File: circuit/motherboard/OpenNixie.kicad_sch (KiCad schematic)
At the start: 29 parts, among them J1 Jack-DC, J2 Nixie_Conn_12P, J3 Nixie_Conn_12P, J4 Nixie_Conn_12P, J5 Nixie_Conn_12P, J6 Conn_01x05, Q1 MPSA42, Q2 TK8P65W, U1 AMS1117, U2 MAX1771CSA, U3 74HC595, U4 74HC595

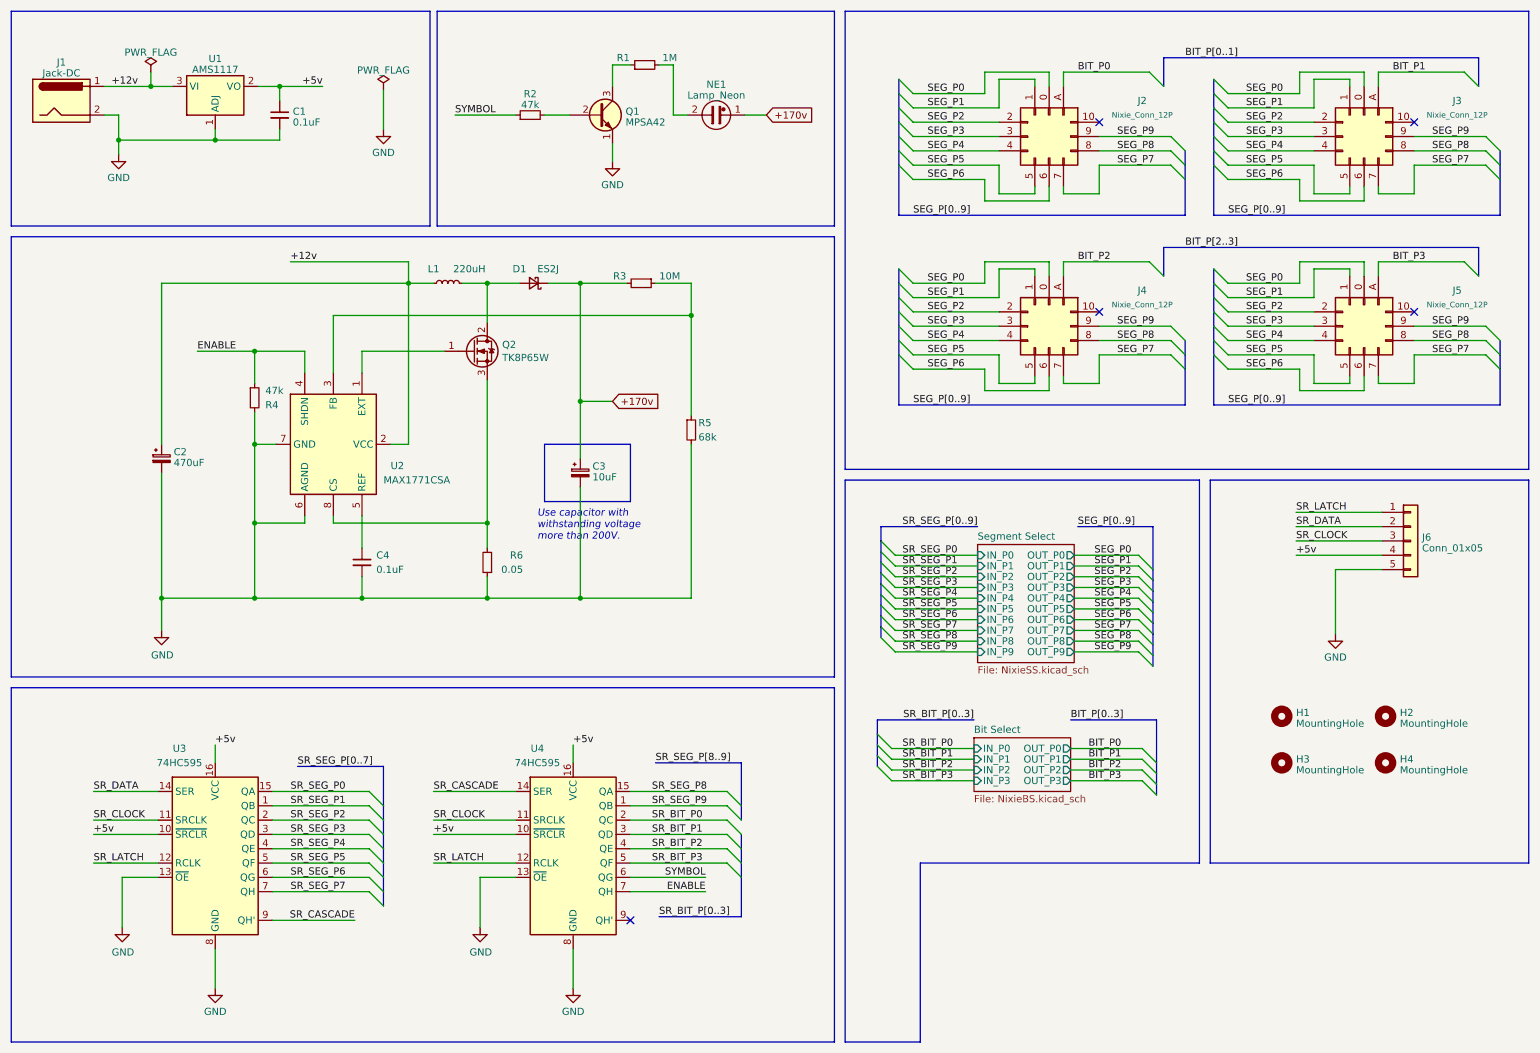
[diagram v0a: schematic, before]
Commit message: Some integration works
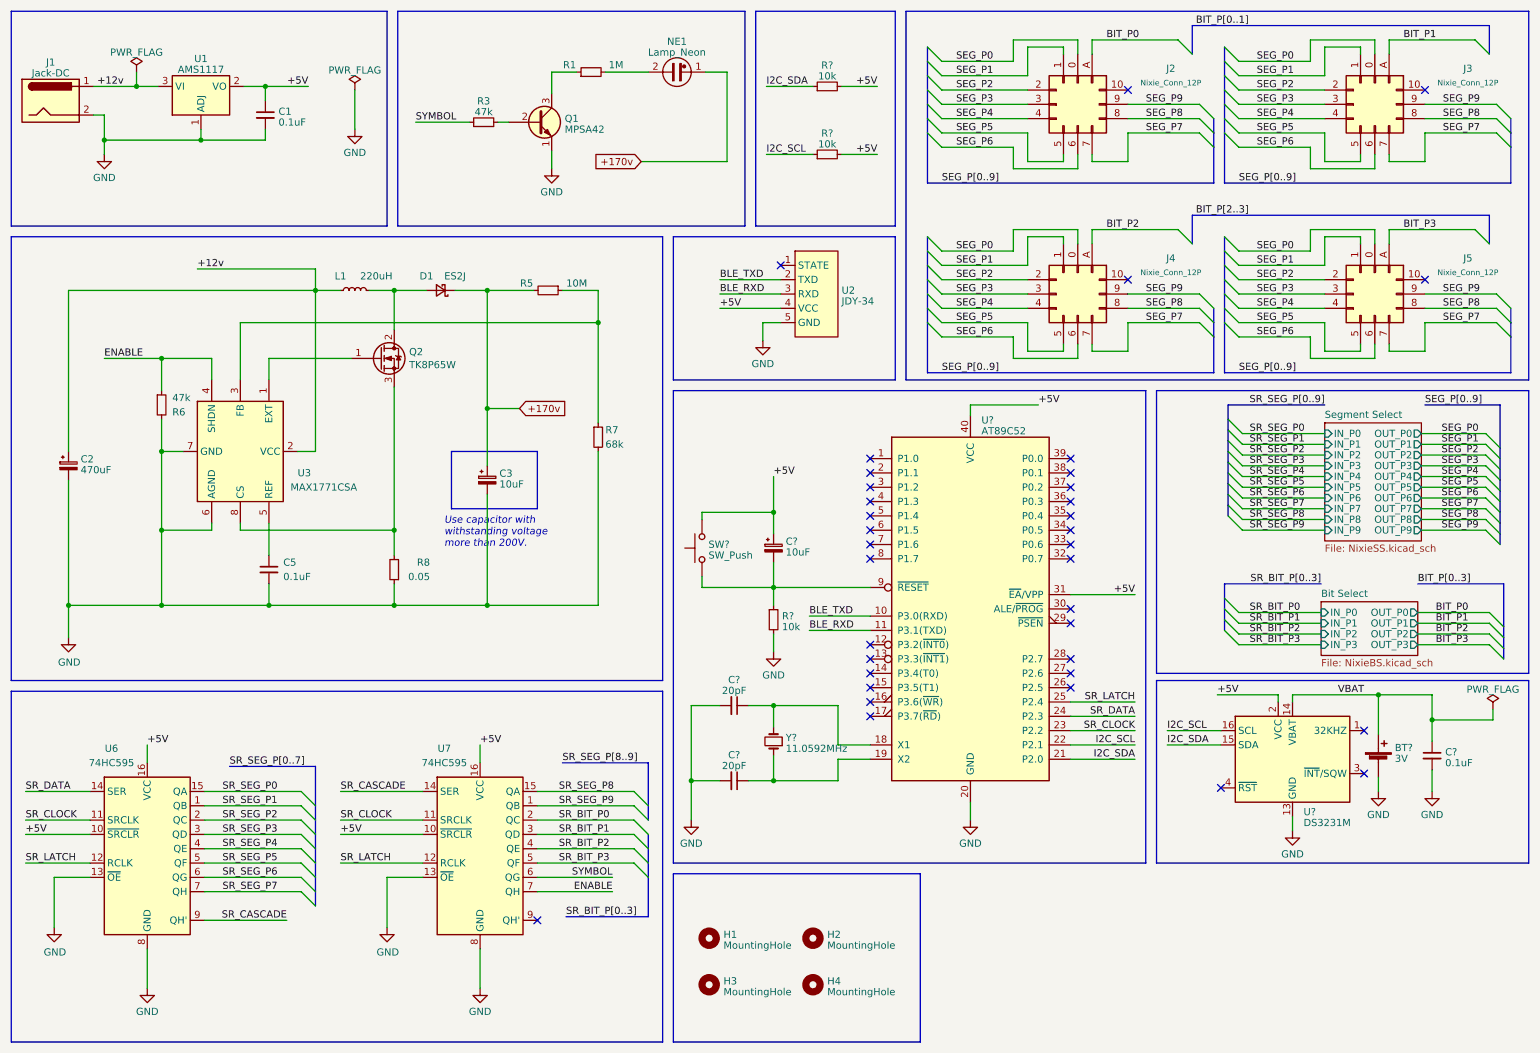
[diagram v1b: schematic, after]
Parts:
- removed J6: Conn_01x05, Connector_PinHeader_2.54mm:PinHeader_1x05_P2.54mm_Vertical, symbol Connector_Generic:Conn_01x05
- added BT?: 3V, Battery:BatteryHolder_LINX_BAT-HLD-012-SMT, symbol Device:Battery_Cell
- added C? (x2): 20pF, Capacitor_THT:C_Disc_D3.0mm_W2.0mm_P2.50mm, symbol Device:C_Small
- added C?: 10uF, Capacitor_THT:CP_Radial_D5.0mm_P2.50mm, symbol Device:C_Polarized_Small
- added C?: 0.1uF, Capacitor_THT:C_Disc_D3.0mm_W2.0mm_P2.50mm, symbol Device:C_Small
- added R? (x3): 10k, Resistor_THT:R_Axial_DIN0204_L3.6mm_D1.6mm_P7.62mm_Horizontal, symbol Device:R_Small
- added SW?: SW_Push, Button_Switch_SMD:SW_SPST_FSMSM, symbol Switch:SW_Push
- added U2: JDY-34, Connector_PinSocket_2.54mm:PinSocket_1x05_P2.54mm_Vertical, symbol Nixie_Clock:JDY-34
- added U?: AT89C52, Package_DIP:DIP-40_W15.24mm, symbol Nixie_Clock:AT89C52
- added U?: DS3231M, Package_SO:SOIC-16W_7.5x10.3mm_P1.27mm, symbol Timer_RTC:DS3231M
- added Y?: 11.0592MHz, Crystal:Crystal_HC18-U_Vertical, symbol Device:Crystal_Small
- R1: footprint Resistor_THT:R_Axial_DIN0204_L3.6mm_D1.6mm_P5.08mm_Horizontal -> Resistor_THT:R_Axial_DIN0204_L3.6mm_D1.6mm_P7.62mm_Horizontal
- R3: renamed from R2; footprint Resistor_THT:R_Axial_DIN0204_L3.6mm_D1.6mm_P5.08mm_Horizontal -> Resistor_THT:R_Axial_DIN0204_L3.6mm_D1.6mm_P7.62mm_Horizontal
- R5: renamed from R3; footprint Resistor_THT:R_Axial_DIN0204_L3.6mm_D1.6mm_P5.08mm_Horizontal -> Resistor_THT:R_Axial_DIN0204_L3.6mm_D1.6mm_P7.62mm_Horizontal
- R6: renamed from R4; footprint Resistor_THT:R_Axial_DIN0204_L3.6mm_D1.6mm_P5.08mm_Horizontal -> Resistor_THT:R_Axial_DIN0204_L3.6mm_D1.6mm_P7.62mm_Horizontal
- R7: renamed from R5; footprint Resistor_THT:R_Axial_DIN0204_L3.6mm_D1.6mm_P5.08mm_Horizontal -> Resistor_THT:R_Axial_DIN0204_L3.6mm_D1.6mm_P7.62mm_Horizontal
- renumbered C4 to C5, R6 to R8, U2 to U3, U3 to U6, U4 to U7
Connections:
- net GND: now also BT?.2 (-), C?.2, C?.2, C?.2, R?.2, U2.5 (GND), U?.10 (GND), U?.11 (GND), U?.12 (GND), U?.13 (GND), U?.20 (GND), U?.5 (GND), U?.6 (GND), U?.7 (GND), U?.8 (GND), U?.9 (GND)
- net SR_CLOCK: now also U?.23 (P2.2)
- net SR_DATA: now also U?.24 (P2.3)
- net SR_LATCH: now also U?.25 (P2.4)
- net +5v renamed +5V
- net +5V: now also C?.1, R?.2, R?.2, SW?.1, U2.4 (VCC), U?.2 (VCC), U?.31 (~{EA}/VPP), U?.40 (VCC)
- new net: C?.2, R?.1, SW?.2, U?.9 (~{RESET})
- new net: C?.1, U?.18 (X1), Y?.2
- new net: C?.1, U?.19 (X2), Y?.1
- new net BLE_RXD: U2.3 (RXD), U?.11 (P3.1(TXD))
- new net BLE_TXD: U2.2 (TXD), U?.10 (P3.0(RXD))
- new net I2C_SCL: R?.1, U?.16 (SCL), U?.22 (P2.1)
- new net I2C_SDA: R?.1, U?.15 (SDA), U?.21 (P2.0)
- new net VBAT: BT?.1 (+), C?.1, U?.14 (VBAT)
- no-connect marks 5 -> 36
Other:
- moved on the sheet: C1, C2, C3, C5, D1, H1, H2, H3, H4, J1, J2, J3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
